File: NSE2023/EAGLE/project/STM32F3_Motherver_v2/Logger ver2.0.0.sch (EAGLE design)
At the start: 36 parts, among them SW1 SRIDE_SWITCH

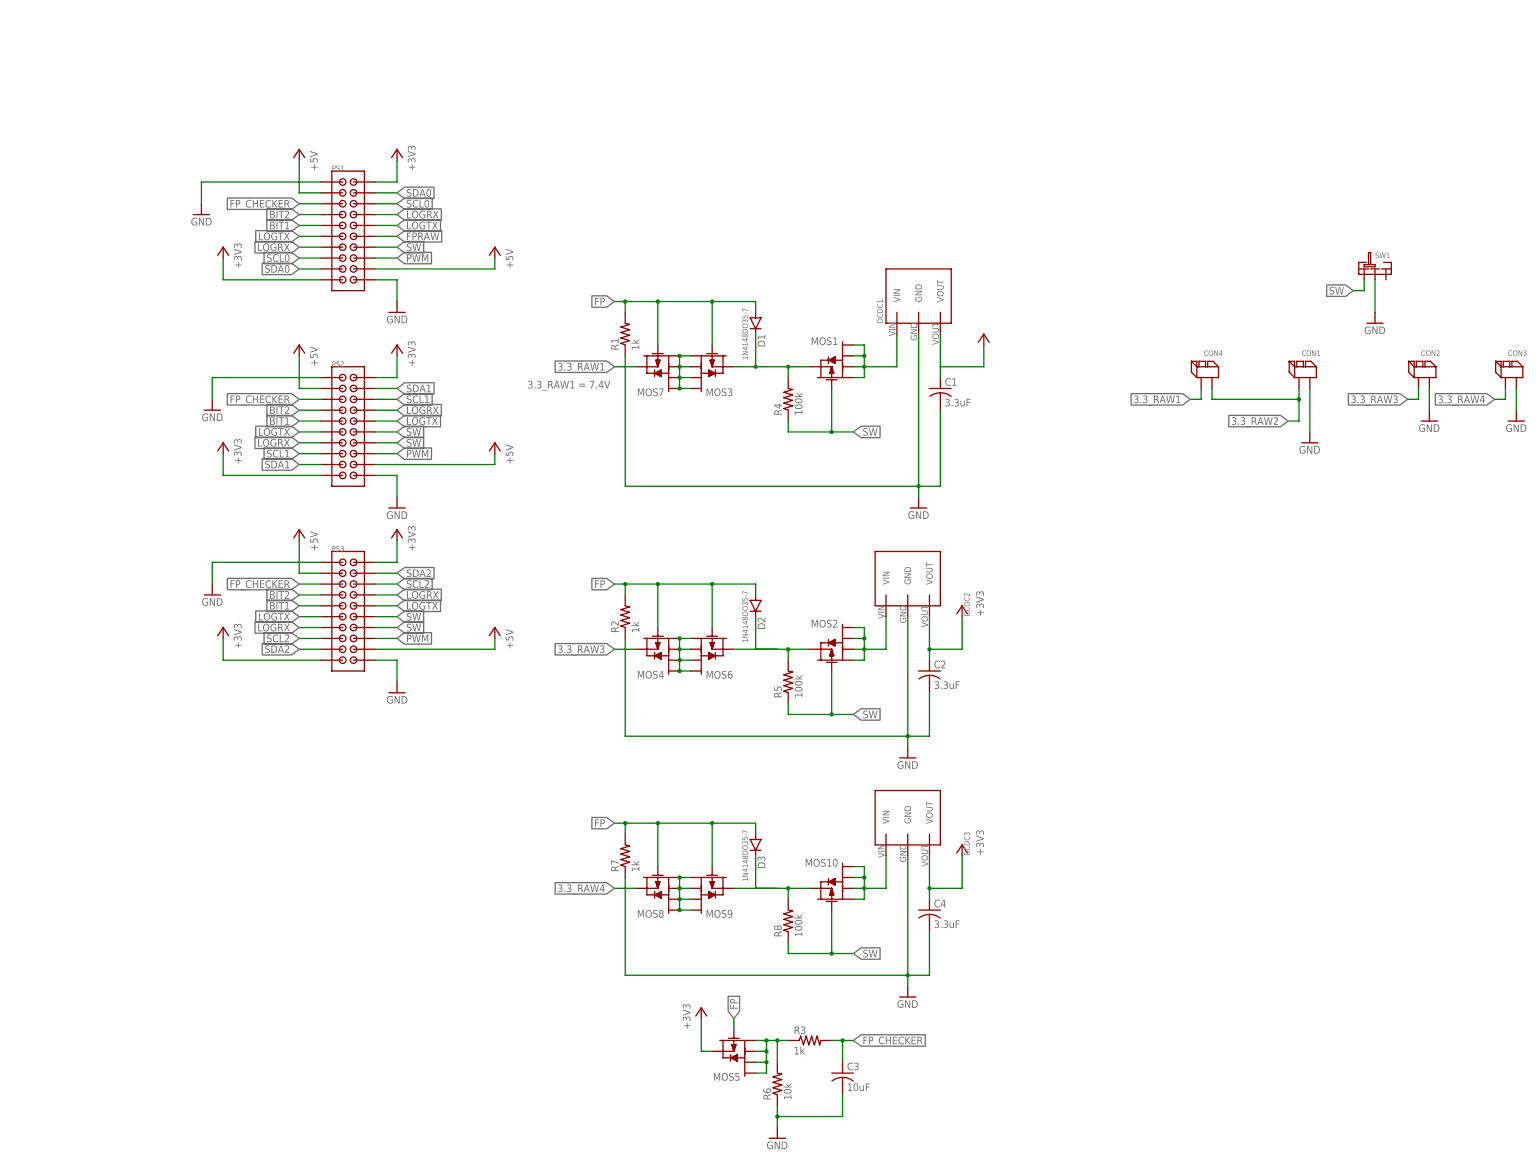
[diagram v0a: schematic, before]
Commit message: create final board NSE2023
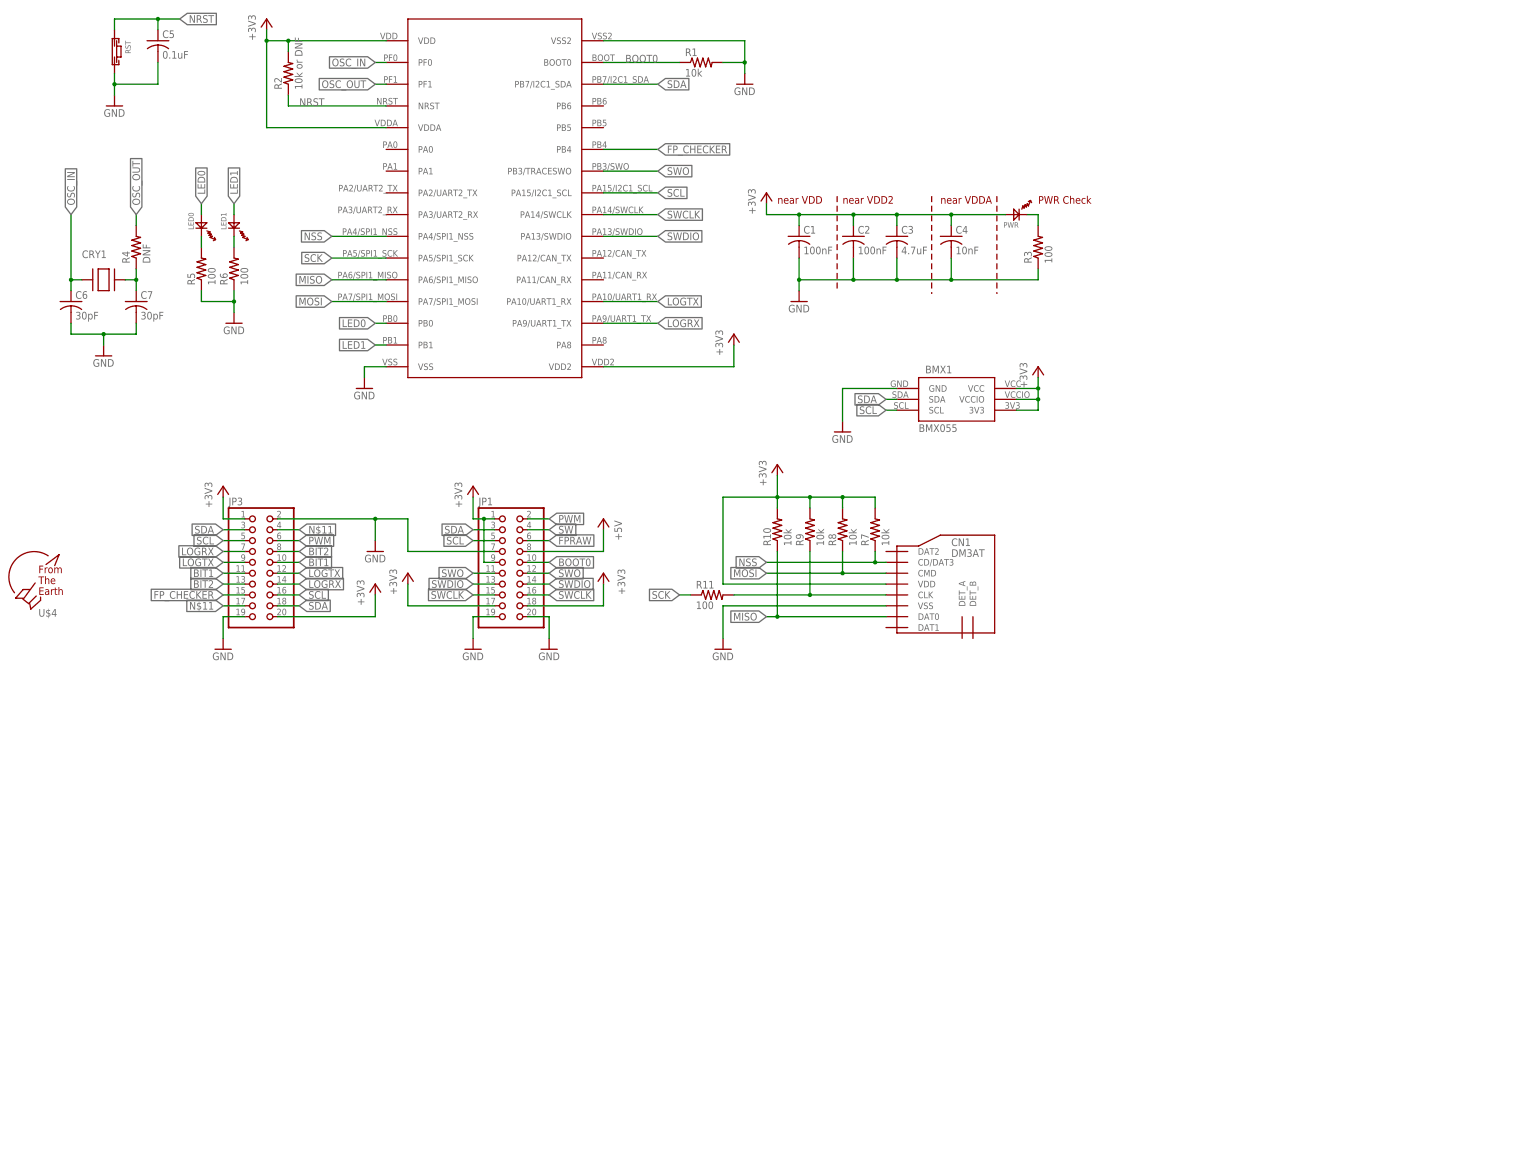
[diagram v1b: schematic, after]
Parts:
- removed CON1, CON2, CON3, CON4: (no value), XR Connector:2PIN
- removed D1, D2, D3: 1N4148DO35-7, diode:1N4148DO35-7
- removed DCDC1: (no value), DC-DC:5V1A_M78AR05-1
- removed DCDC2, DCDC3: (no value), DC-DC:3.3V1A_M78AR033-1
- removed MOS1, MOS10, MOS2, MOS3, MOS4, MOS5, MOS6, MOS7, MOS8, MOS9: (no value), Chip MOSFET:PCH_SSM6J808R
- removed PS1, PS2, PS3: (no value), PinSocket:2X10
- removed SW1: SRIDE_SWITCH, Sride Switch:SRIDE_SWITCH
- added BMX1: BMX055, BMX055:BMX055
- added C5: 0.1uF, rcl:C-USC1608
- added C6, C7: 30pF, rcl:C-USC1608
- added CN1: DM3AT, microSD:DM3AT
- added CRY1: (no value), Crystal:8MHZ
- added JP1, JP3: (no value), pinhead:PINHD-2X10/90
- added LED0, LED1, PWR: (no value), Chip LED:OSXX1608C1A
- added R10, R9: 10k, rcl:R-US_R0603
- added R11: 100, rcl:R-US_R0603
- added RST: (no value), Tact switch:TVAF06-A020B-R
- added U$1: STM32F303K8, STM32F303K8:STM32F303K8
- added U$4: F.T.E.LOGO, logo:F.T.E.LOGO
- C1, C2: value 3.3uF -> 100nF; device rcl:C-USC0603 -> rcl:C-USC1608
- C3: value 10uF -> 4.7uF; device rcl:C-USC0603 -> rcl:C-USC1608
- C4: value 3.3uF -> 10nF; device rcl:C-USC0603 -> rcl:C-USC1608
- R1, R7: value 1k -> 10k
- R2: value 1k -> 10k or DNF
- R3: value 1k -> 100
- R4: value 100k -> DNF
- R5: value 100k -> 100
- R6: value 10k -> 100
- R8: value 100k -> 10k
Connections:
- removed net +5V1: DCDC1.VIN, MOS1.1, MOS1.2, MOS1.5, MOS1.6
- removed net 3.3_RAW1: CON4.P$2, MOS7.4
- removed net 3.3_RAW2: CON1.P$2, CON4.P$1
- removed net 3.3_RAW3: CON2.P$2, MOS4.4
- removed net 3.3_RAW4: CON3.P$2, MOS8.4
- removed net FP: D1.A, D2.A, D3.A, MOS3.3, MOS4.3, MOS5.3, MOS6.3, MOS7.3, MOS8.3, MOS9.3, R1.2, R2.2, R7.2
- removed net N$12: MOS3.1, MOS3.2, MOS3.5, MOS3.6, MOS7.1, MOS7.2, MOS7.5, MOS7.6
- removed net N$14: MOS5.1, MOS5.2, MOS5.5, MOS5.6, R3.1, R6.2
- removed net N$5: DCDC2.VIN, MOS2.1, MOS2.2, MOS2.5, MOS2.6
- removed net N$6: DCDC3.VIN, MOS10.1, MOS10.2, MOS10.5, MOS10.6
- removed net SCL0: PS1.P$15, PS1.P$6
- removed net SCL1: PS2.P$15, PS2.P$6
- removed net SCL2: PS3.P$15, PS3.P$6
- removed net SDA0: PS1.P$17, PS1.P$4
- removed net SDA1: PS2.P$17, PS2.P$4
- removed net SDA2: PS3.P$17, PS3.P$4
- new net BOOT0: JP1.10, R1.1, U$1.BOOT0
- new net LED0: LED0.AN, U$1.PB0
- new net LED1: LED1.AN, U$1.PB1
- new net MISO: CN1.DAT0, R10.1, U$1.PA6/SPI1_MISO
- new net MOSI: CN1.CMD, R8.1, U$1.PA7/SPI1_MOSI
- new net N$7: CN1.CLK, R11.2, R9.1
- new net NRST: C5.1, R2.1, RST.P$1, U$1.NRST
- new net NSS: CN1.CD/DAT3, R7.1, U$1.PA4/SPI1_NSS
- new net OSC_IN: C6.1, CRY1.P$1, U$1.PF0
- new net OSC_OUT: R4.2, U$1.PF1
- new net SCK: R11.1, U$1.PA5/SPI1_SCK
- new net SCL: BMX1.SCL, JP1.5, JP3.16, JP3.5, U$1.PA15/I2C1_SCL
- new net SDA: BMX1.SDA, JP1.3, JP3.18, JP3.3, U$1.PB7/I2C1_SDA
- new net SWCLK: JP1.15, JP1.16, U$1.PA14/SWCLK
- new net SWDIO: JP1.13, JP1.14, U$1.PA13/SWDIO
- new net SWO: JP1.11, JP1.12, U$1.PB3/TRACESWO
- net +3V3: now also BMX1.3V3, BMX1.VCC, BMX1.VCCIO, C1.1, C3.1, CN1.VDD, JP1.1, JP1.17, JP1.18, JP1.9, JP3.1, JP3.20, PWR.AN, R10.2, R2.2, R7.2, R8.2, R9.2, U$1.VDD, U$1.VDD2, U$1.VDDA; no longer DCDC2.VOUT, DCDC3.VOUT, MOS5.4, PS1.P$19, PS1.P$2, PS2.P$19, PS2.P$2, PS3.P$19, PS3.P$2
- net +5V: now also JP1.8; no longer C1.1, DCDC1.VOUT, PS1.P$18, PS1.P$3, PS2.P$18, PS2.P$3, PS3.P$18, PS3.P$3
- net BIT1: now also JP3.10, JP3.11; no longer PS1.P$9, PS2.P$9, PS3.P$9
- net BIT2: now also JP3.13, JP3.8; no longer PS1.P$7, PS2.P$7, PS3.P$7
- net FPRAW: now also JP1.6; no longer PS1.P$12
- net FP_CHECKER: now also JP3.15, U$1.PB4; no longer C3.1, PS1.P$5, PS2.P$5, PS3.P$5, R3.2
- net GND: now also BMX1.GND, C5.2, C6.2, C7.2, CN1.VSS, JP1.19, JP1.20, JP1.7, JP3.19, JP3.2, R1.2, R3.1, R5.1, RST.P$2, U$1.VSS, U$1.VSS2; no longer CON1.P$1, CON2.P$1, CON3.P$1, DCDC1.GND, DCDC2.GND, DCDC3.GND, PS1.P$1, PS1.P$20, PS2.P$1, PS2.P$20, PS3.P$1, PS3.P$20, R1.1, R2.1, R7.1, SW1.LR
- net LOGRX: now also JP3.14, JP3.7, U$1.PA9/UART1_TX; no longer PS1.P$13, PS1.P$8, PS2.P$13, PS2.P$8, PS3.P$13, PS3.P$8
- net LOGTX: now also JP3.12, JP3.9, U$1.PA10/UART1_RX; no longer PS1.P$10, PS1.P$11, PS2.P$10, PS2.P$11, PS3.P$10, PS3.P$11
- net N$1: now also PWR.CT, R3.2; no longer D2.C, MOS2.4, MOS6.4, R5.2
- net N$11: now also JP3.17, JP3.4; no longer D1.C, MOS1.4, MOS3.4, R4.2
- net N$2: now also LED0.CT, R5.2; no longer MOS4.1, MOS4.2, MOS4.5, MOS4.6, MOS6.1, MOS6.2, MOS6.5, MOS6.6
- net N$3: now also C7.1, CRY1.P$2, R4.1; no longer D3.C, MOS10.4, MOS9.4, R8.2
- net N$4: now also LED1.CT, R6.2; no longer MOS8.1, MOS8.2, MOS8.5, MOS8.6, MOS9.1, MOS9.2, MOS9.5, MOS9.6
- net PWM: now also JP1.2, JP3.6; no longer PS1.P$16, PS2.P$16, PS3.P$16
- net SW: now also JP1.4; no longer MOS1.3, MOS10.3, MOS2.3, PS1.P$14, PS2.P$12, PS2.P$14, PS3.P$12, PS3.P$14, R4.1, R5.1, R8.1, SW1.L
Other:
- note added: "PWR Check"
- note added: "near VDD"
- note added: "near VDD2"
- note added: "near VDDA"
- note removed: "3.3_RAW1 = 7.4V"
- moved on the sheet: C1, C2, C3, C4, R1, R2, R3, R4, R5, R6, R7, R8
